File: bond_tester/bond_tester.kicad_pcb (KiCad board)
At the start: 2 copper layers, 40 x 100 mm, 5 parts

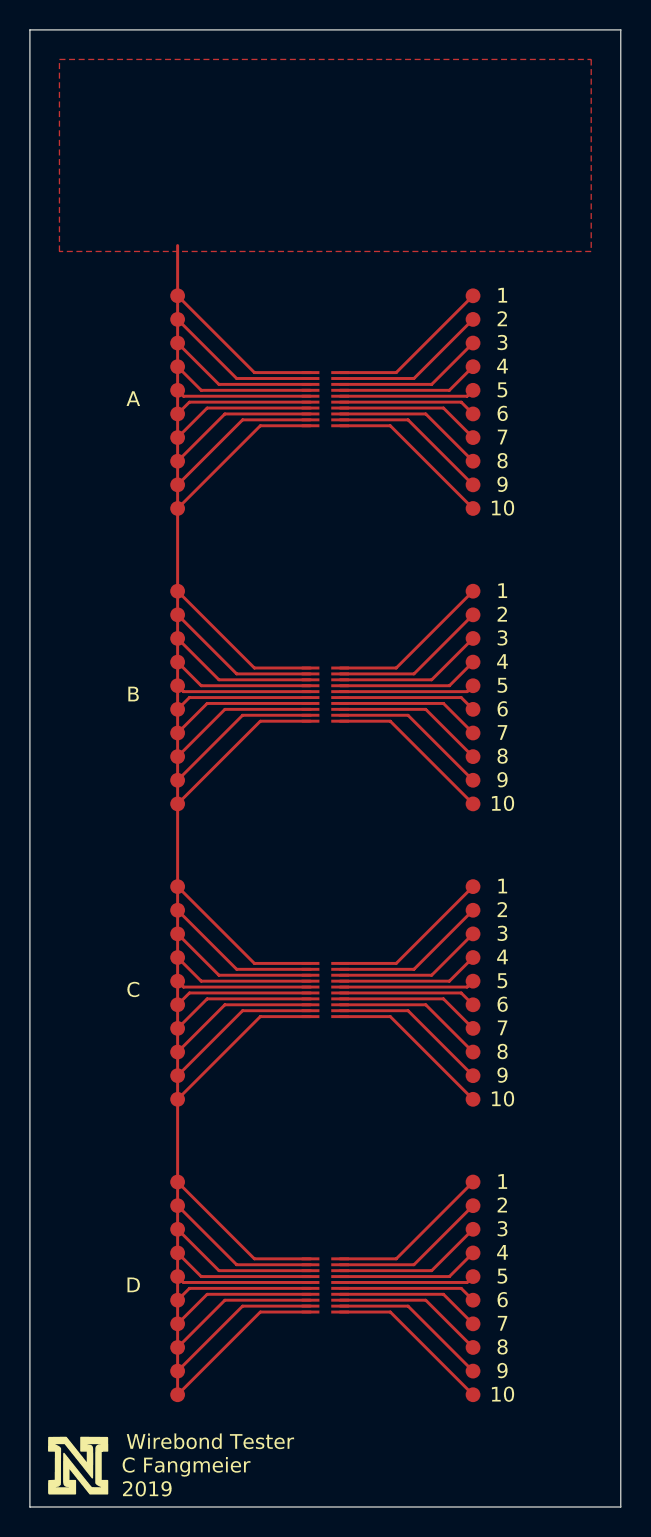
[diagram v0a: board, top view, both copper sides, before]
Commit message: Rev bond_tester
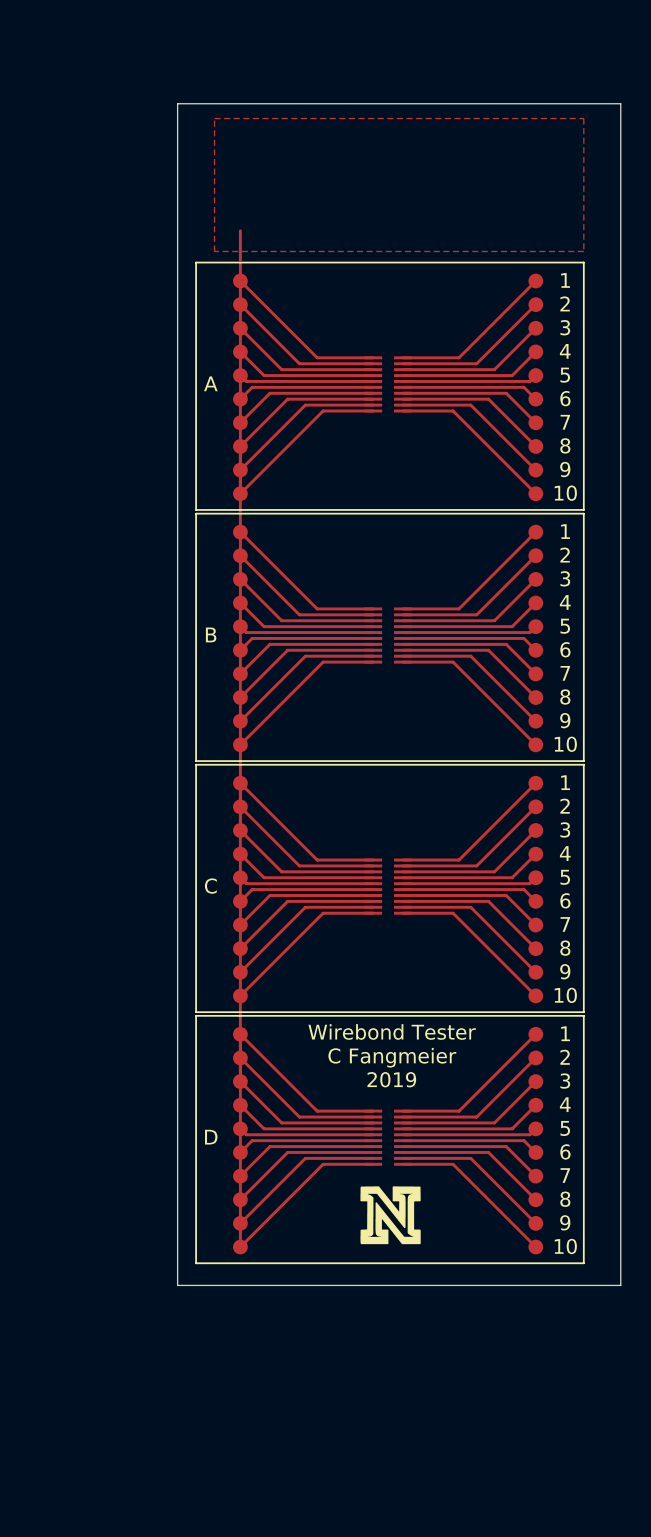
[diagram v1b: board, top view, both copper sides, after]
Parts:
- moved G*** 27.1 mm to (108.8, 115.2)
- moved D 10.9 mm to (109.2, 110.0)
- moved C 8.19 mm to (109.2, 93.0)
- moved B 5.84 mm to (109.2, 76.0)
- moved A 4.37 mm to (109.2, 59.0)
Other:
- board size 40 x 100 mm -> 30 x 80 mm
- board text added: "Wirebond Tester C Fangmeier 2019"
- board text removed: "C Fangmeier 2019"
- board text removed: "Wirebond Tester"
